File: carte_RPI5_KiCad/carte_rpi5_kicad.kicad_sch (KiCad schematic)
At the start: 31 parts, among them J1 Conn_01x03, J10 RPI5_40pins, J2 Conn_01x03, J3 Conn_01x03, J4 Conn_01x03, J5 Conn_01x03, J6 Conn_01x03, J7 Conn_01x03, J8 Conn_01x03, J9 XT60-M, SW1 SW_SPDT

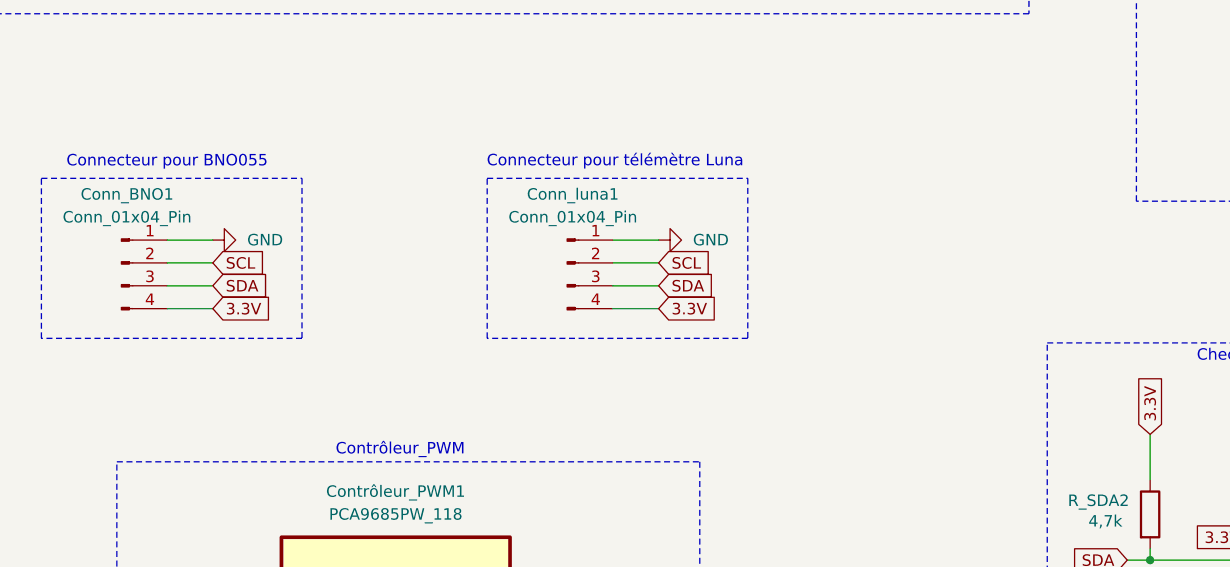
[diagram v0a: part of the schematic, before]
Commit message: Modif_carte_elec
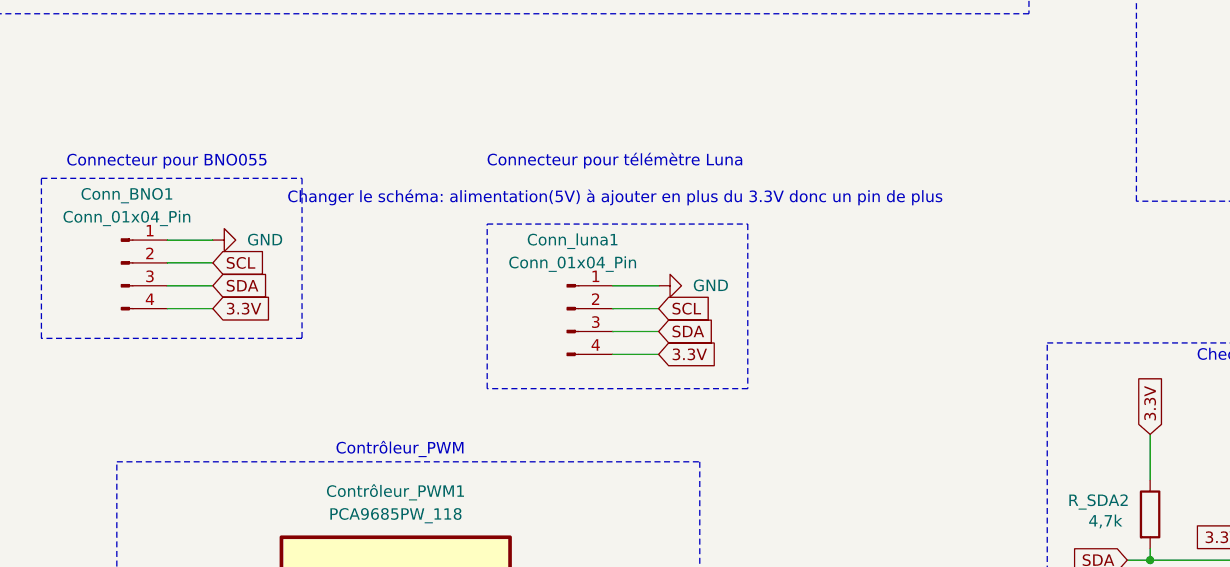
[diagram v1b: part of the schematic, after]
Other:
- note added: "Connecteur pour télémètre Luna Changer le schéma: alimentation(5V) à ajouter en plus du 3.3V donc un pin de plus"
- note removed: "Connecteur pour télémètre Luna"
- moved on the sheet: Conn_luna1
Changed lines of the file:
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@@
 	)
 	(rectangle
-		(start 120.396 97.536)
-		(end 120.396 97.536)
+		(start 120.396 102.616)
+		(end 120.396 102.616)
 		(stroke
 			(width 0)
@@
 	)
 	(rectangle
-		(start 91.44 80.772)
-		(end 120.396 98.552)
+		(start 91.44 85.852)
+		(end 120.396 104.14)
 		(stroke
 			(width 0)
@@
 		)
 	)
-	(text "Connecteur pour télémètre Luna\n\n\n"
+	(text "Connecteur pour télémètre Luna\n\nChanger le schéma: alimentation(5V) à ajouter en plus du 3.3V donc un pin de plus\n"
 		(exclude_from_sim no)
 		(at 105.664 81.026 0)
@@
 	(wire
 		(pts
-			(xy 105.41 92.71) (xy 110.49 92.71)
+			(xy 105.41 97.79) (xy 110.49 97.79)
 		)
 		(stroke
@@
 	(wire
 		(pts
-			(xy 105.41 90.17) (xy 110.49 90.17)
+			(xy 105.41 95.25) (xy 110.49 95.25)
 		)
 		(stroke
@@
 	(wire
 		(pts
-			(xy 105.41 95.25) (xy 110.49 95.25)
+			(xy 105.41 100.33) (xy 110.49 100.33)
 		)
 		(stroke
@@
 	(wire
 		(pts
-			(xy 105.41 87.63) (xy 110.49 87.63)
+			(xy 105.41 92.71) (xy 110.49 92.71)
 		)
 		(stroke
@@
 	(global_label "3.3V"
 		(shape input)
-		(at 110.49 95.25 0)
+		(at 110.49 100.33 0)
 		(fields_autoplaced yes)
 		(effects
@@
 		)
 		(property "Intersheetrefs" "${INTERSHEET_REFS}"
-			(at 117.5876 95.25 0)
+			(at 117.5876 100.33 0)
 			(effects
 				(font
@@
 	(global_label "SCL"
 		(shape input)
-		(at 110.49 90.17 0)
+		(at 110.49 95.25 0)
 		(fields_autoplaced yes)
 		(effects
@@
 		)
 		(property "Intersheetrefs" "${INTERSHEET_REFS}"
-			(at 116.9828 90.17 0)
+			(at 116.9828 95.25 0)
 			(effects
 				(font
@@
 	(global_label "SDA"
 		(shape input)
-		(at 110.49 92.71 0)
+		(at 110.49 97.79 0)
 		(fields_autoplaced yes)
 		(effects
@@
 		)
 		(property "Intersheetrefs" "${INTERSHEET_REFS}"
-			(at 117.0433 92.71 0)
+			(at 117.0433 97.79 0)
 			(effects
 				(font
@@
 	(symbol
 		(lib_id "power:GND")
-		(at 110.49 87.63 90)
+		(at 110.49 92.71 90)
 		(unit 1)
 		(exclude_from_sim no)
@@
 		(fields_autoplaced yes)
 		(property "Reference" "#PWR019"
-			(at 116.84 87.63 0)
+			(at 116.84 92.71 0)
 			(effects
 				(font
@@
 		)
 		(property "Value" "GND"
-			(at 114.3 87.6299 90)
+			(at 114.3 92.7099 90)
 			(effects
 				(font
@@
 		)
 		(property "Footprint" ""
-			(at 110.49 87.63 0)
+			(at 110.49 92.71 0)
 			(effects
 				(font
@@
 		)
 		(property "Datasheet" ""
-			(at 110.49 87.63 0)
+			(at 110.49 92.71 0)
 			(effects
 				(font
@@
 		)
 		(property "Description" "Power symbol creates a global label with name \"GND\" , ground"
-			(at 110.49 87.63 0)
+			(at 110.49 92.71 0)
 			(effects
 				(font
@@
 	(symbol
 		(lib_id "Connector:Conn_01x04_Pin")
-		(at 100.33 90.17 0)
+		(at 100.33 95.25 0)
 		(unit 1)
 		(exclude_from_sim no)
@@
 		(fields_autoplaced yes)
 		(property "Reference" "Conn_luna1"
-			(at 100.965 82.55 0)
+			(at 100.965 87.63 0)
 			(effects
 				(font
@@
 		)
 		(property "Value" "Conn_01x04_Pin"
-			(at 100.965 85.09 0)
+			(at 100.965 90.17 0)
 			(effects
 				(font
@@
 		)
 		(property "Footprint" "Connector_PinSocket_2.54mm:PinSocket_1x04_P2.54mm_Vertical"
-			(at 100.33 90.17 0)
+			(at 100.33 95.25 0)
 			(effects
 				(font
@@
 		)
 		(property "Datasheet" "~"
-			(at 100.33 90.17 0)
+			(at 100.33 95.25 0)
 			(effects
 				(font
@@
 		)
 		(property "Description" "Generic connector, single row, 01x04, script generated"
-			(at 100.33 90.17 0)
+			(at 100.33 95.25 0)
 			(effects
 				(font

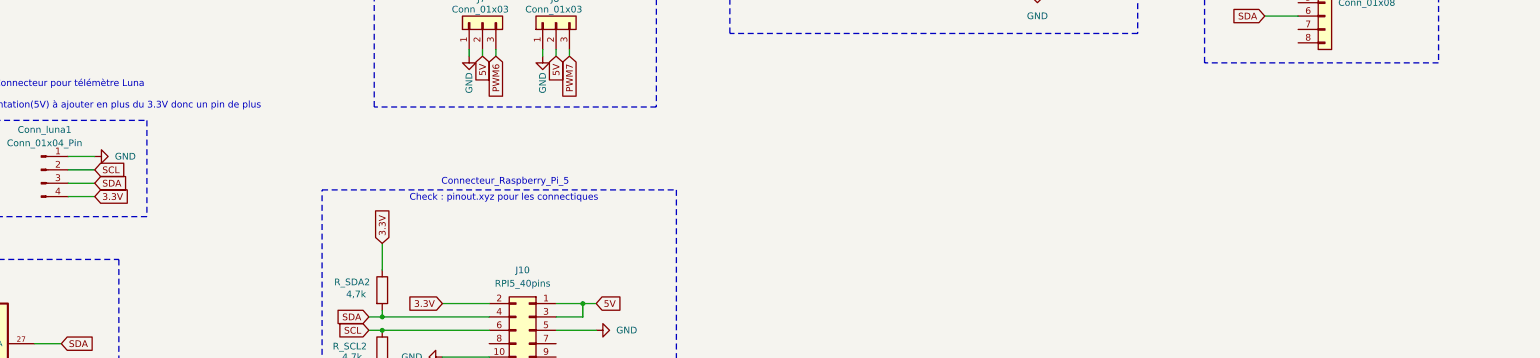
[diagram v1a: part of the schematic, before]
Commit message: mise à  jour
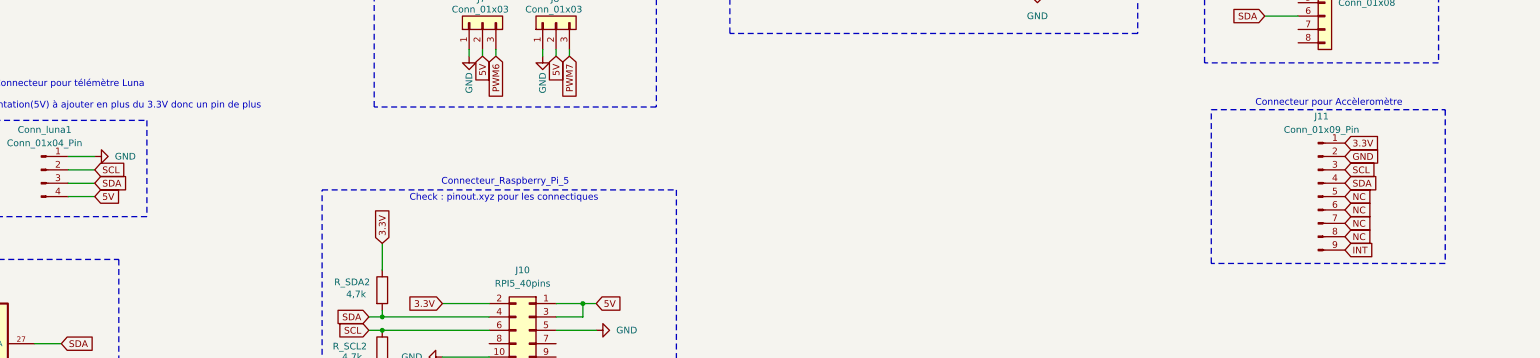
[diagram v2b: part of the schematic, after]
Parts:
- added J11: Conn_01x09_Pin, symbol Connector:Conn_01x09_Pin
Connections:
- net 3.3V: now also J11.1 (Pin_1); no longer Conn_luna1.4 (Pin_4)
- net 5V: now also Conn_luna1.4 (Pin_4)
- net GND: now also J11.2 (Pin_2)
- net SCL: now also J11.3 (Pin_3)
- net SDA: now also J11.4 (Pin_4)
- new net INT: J11.9 (Pin_9)
- new net NC: J11.5 (Pin_5), J11.6 (Pin_6), J11.7 (Pin_7), J11.8 (Pin_8)
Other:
- note added: "Connecteur pour Accèleromètre"

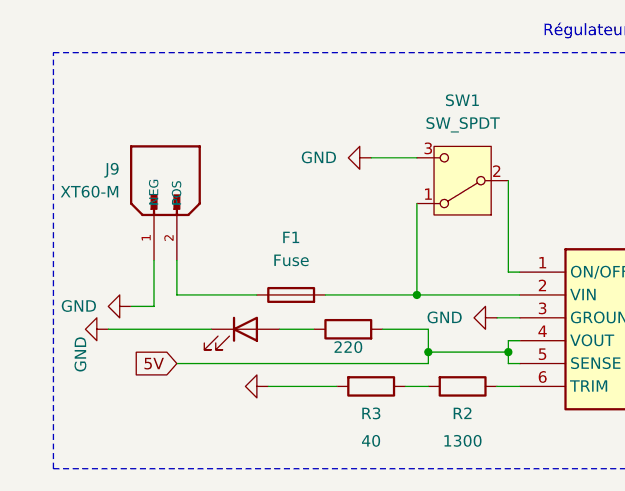
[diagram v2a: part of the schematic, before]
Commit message: maj
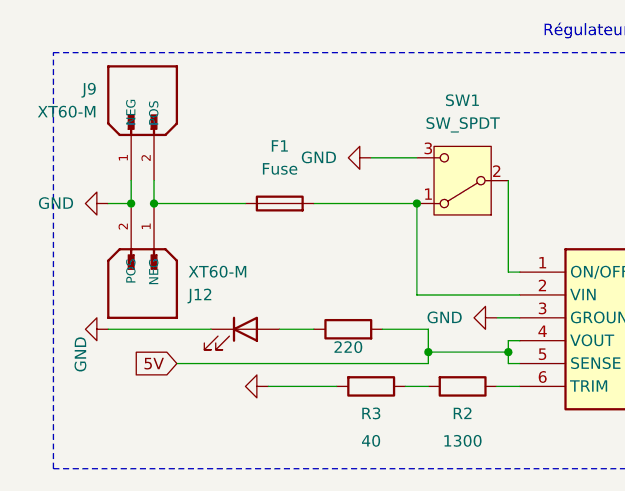
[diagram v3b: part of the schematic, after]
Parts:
- added J12: XT60-M, Connector_AMASS:AMASS_XT60-F_1x02_P7.20mm_Vertical, symbol Librairie_symbole:XT60-M
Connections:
- net GND: now also J12.2 (POS)
- net at F1.1, J9.2 (POS): now also J12.1 (NEG)
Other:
- moved on the sheet: F1, J9

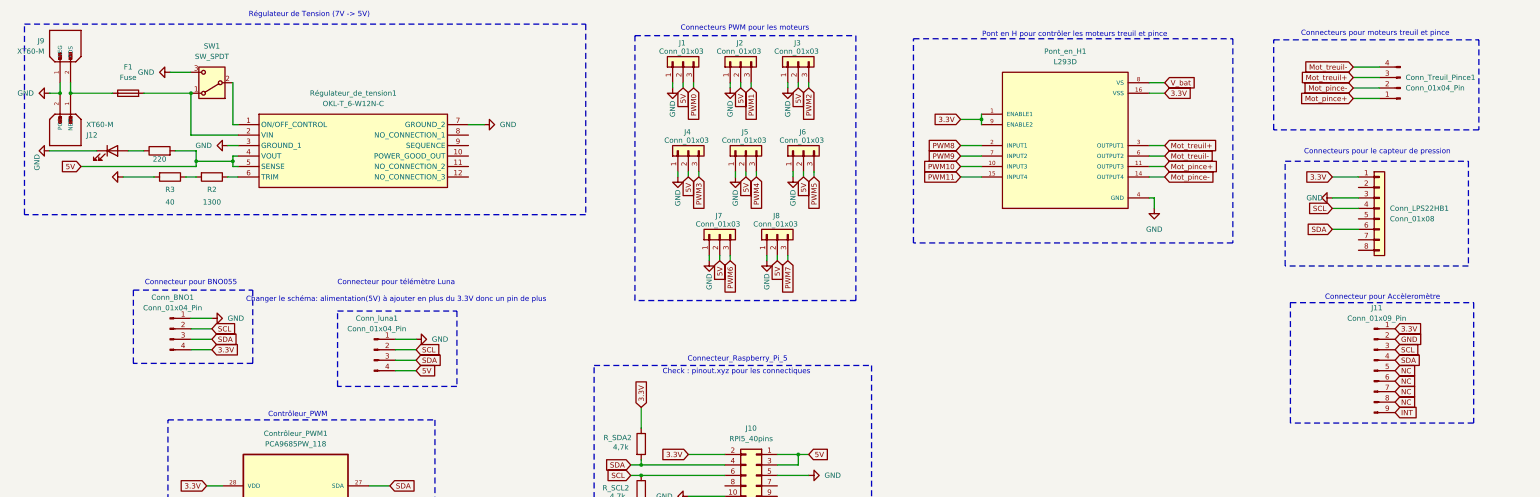
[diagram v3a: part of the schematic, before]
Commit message: maj carte
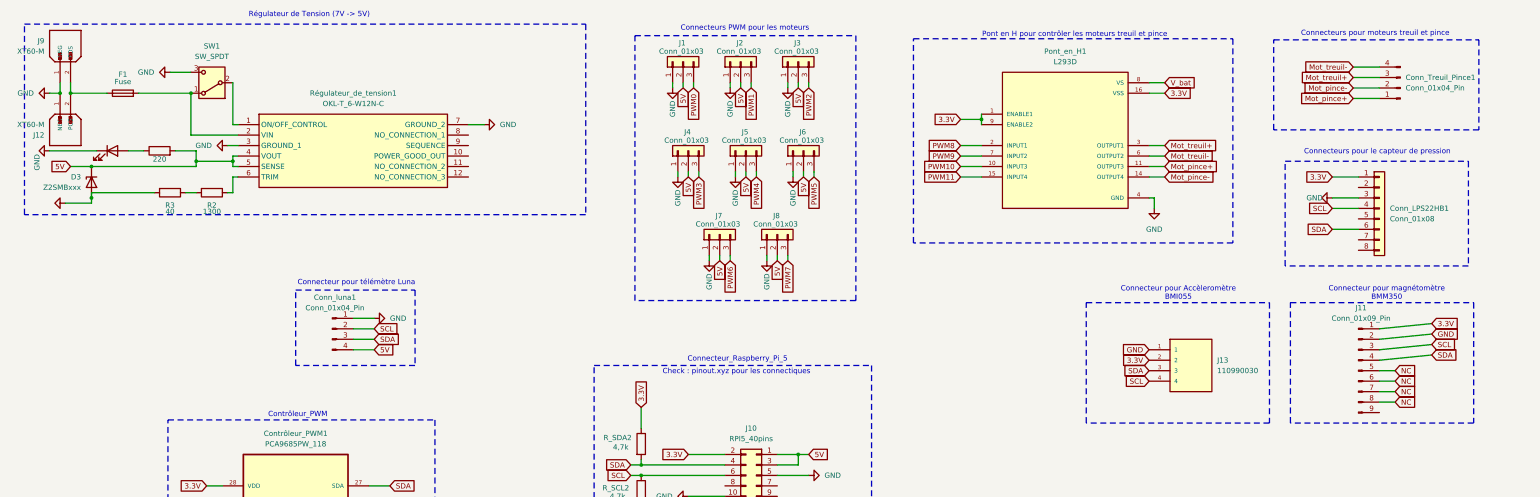
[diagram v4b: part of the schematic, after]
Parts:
- removed Conn_BNO1: Conn_01x04_Pin, Connector_PinSocket_2.54mm:PinSocket_1x04_P2.54mm_Vertical, symbol Connector:Conn_01x04_Pin
- added D3: Z2SMBxxx, Diode_SMD:D_SMB, symbol Diode:Z2SMBxxx
- added J13: 110990030, Connector:NS-Tech_Grove_1x04_P2mm_Vertical, symbol Librairie_symbole:110990030
- F1: footprint librairie_empreintes:PTF-50 -> Fuse:Fuse_1206_3216Metric
- J11: footprint (none) -> Connector_PinSocket_2.54mm:PinSocket_1x09_P2.54mm_Vertical
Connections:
- net 3.3V: now also J13.2
- net 5V: now also D3.1 (K)
- net GND: now also J12.1 (NEG), D3.2 (A), J13.1; no longer J12.2 (POS)
- net SCL: now also J13.4
- net SDA: now also J13.3
- net at F1.1, J9.2 (POS): now also J12.2 (POS); no longer J12.1 (NEG)
- net INT: no longer names the net of J11.9 (Pin_9)
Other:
- note added: "Connecteur pour Accèleromètre BMI055"
- note added: "Connecteur pour magnétomètre BMM350"
- note added: "Connecteur pour télémètre Luna"
- note removed: "Connecteur pour Accèleromètre"
- note removed: "Connecteur pour BNO055"
- note removed: "Connecteur pour télémètre Luna Changer le schéma: alimentation(5V) à ajouter en plus du 3.3V donc un pin de plus"
- moved on the sheet: Conn_luna1, F1, J12, R2, R3
